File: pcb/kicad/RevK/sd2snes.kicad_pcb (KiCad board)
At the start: 2 copper layers, 101.5 x 83 mm, 148 parts, among them J101 SNESCART_EXT, J411 Hirose DM1AA, J421 USB Mini-B SMT, P113 CONN_1, P401 CONN_7X2, P402 CONN_2, P403 CONN_2, P404 CONN_3X2, Q101 2N2222A, Q301 IRLML6402PbF, Q511 2N2222A, U101 74ALVC164245DGG, U102 74ALVC164245DGG, U103 74ALVC164245DGG, U201 XC3S400-PQ208, U230 TS9222, U301 MIC23250-S4YMT, U311 MCP1824-1802E/OT, U321 MCP1824-2502E/OT, U331 PIC12F629-I/P, U341 CS4344, U401 LPC1754, U501 MT45W8MW16, U511 CY62148EV30-ZSXI, X401 12MHz, X402 32.768kHz

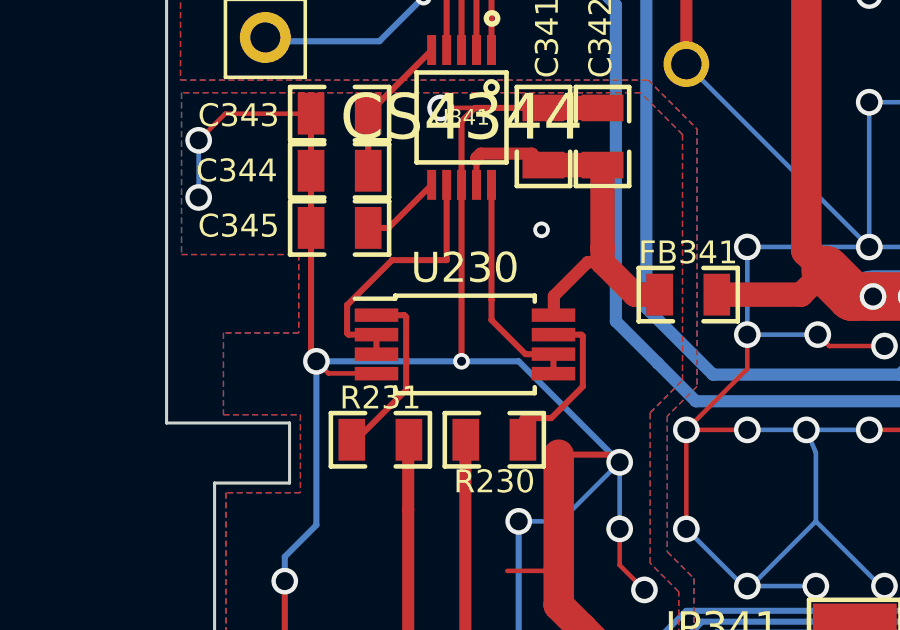
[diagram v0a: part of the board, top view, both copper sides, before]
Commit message: Fix stupid layout mistake
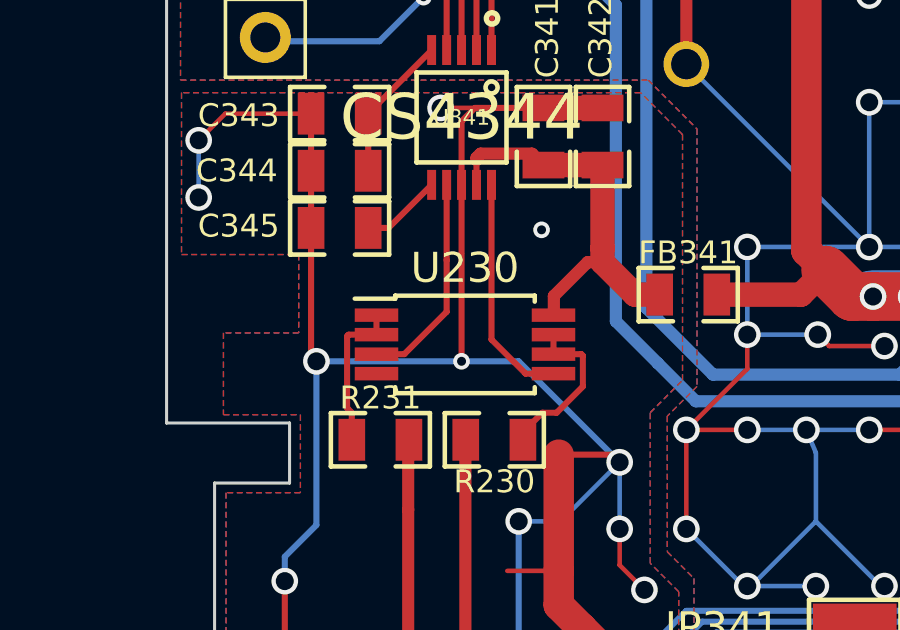
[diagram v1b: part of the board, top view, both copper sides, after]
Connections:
- U230 pad 2: Net-(U230-Pad2) -> Net-(R231-Pad1)
- U230 pad 3: Net-(U230-Pad2) -> Net-(U230-Pad3)
- U230 pad 6: Net-(U230-Pad5) -> Net-(R230-Pad1)
- U341 pad 7: Net-(U230-Pad2) -> Net-(U230-Pad3)
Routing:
- net Net-(U230-Pad2): track 9.03 -> 0.00 mm
- net Net-(U230-Pad3): track 0.00 -> 7.15 mm
- net GNDA: track 106.7 -> 104.5 mm
- net Net-(R231-Pad1): track 6.80 -> 6.18 mm
